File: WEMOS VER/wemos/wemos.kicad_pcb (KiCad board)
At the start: 2 copper layers, 50 x 50 mm, 15 parts, among them J1 9V BATT, J2 MOTOR 1, J3 MOTOR 2, SW1 RESET, SW2 ON/OFF, U1 WeMos D1 Mini, U2 L7805, U3 L293D

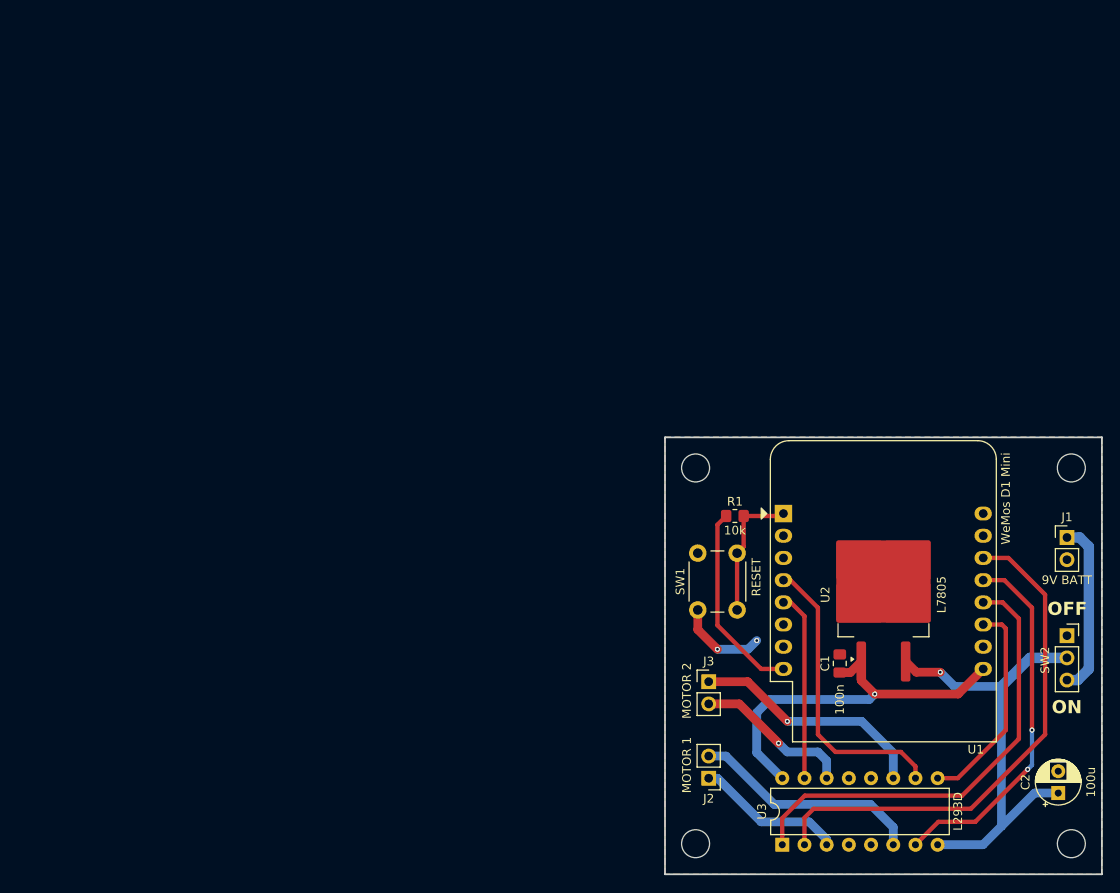
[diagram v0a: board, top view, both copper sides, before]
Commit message: A LOT OF WORK
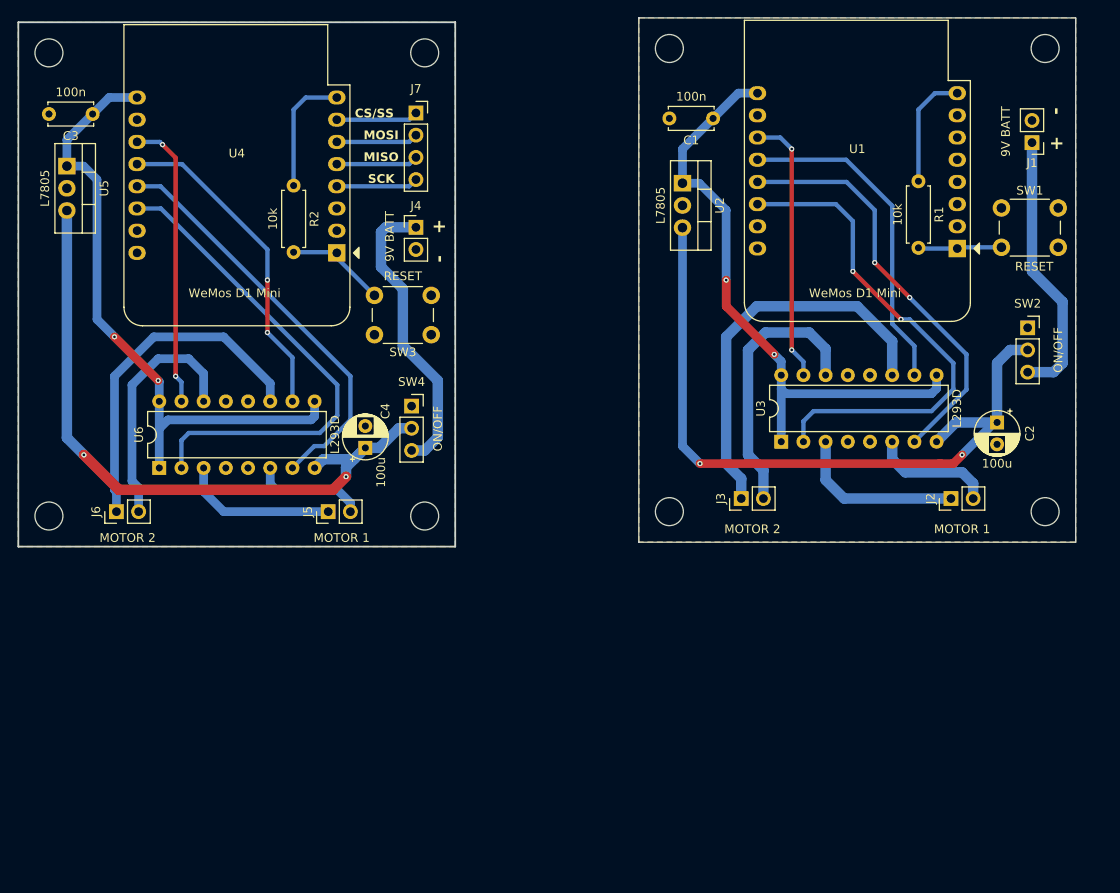
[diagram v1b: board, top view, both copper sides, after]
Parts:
- added C3: 100n, Capacitor_THT:C_Disc_D5.0mm_W2.5mm_P5.00mm, F.Cu at (49.5, 48.0)
- added C4: 100u, Capacitor_THT:CP_Radial_D5.0mm_P2.50mm, F.Cu at (80.7, 86.2)
- added H5: MountingHole, MountingHole:MountingHole_3.2mm_M3, F.Cu at (44.5, 41.0)
- added H6: MountingHole, MountingHole:MountingHole_3.2mm_M3, F.Cu at (87.5, 41.0)
- added H7: MountingHole, MountingHole:MountingHole_3.2mm_M3, F.Cu at (44.5, 94.0)
- added H8: MountingHole, MountingHole:MountingHole_3.2mm_M3, F.Cu at (87.5, 94.0)
- added J4: 9V BATT, Connector_PinHeader_2.54mm:PinHeader_1x02_P2.54mm_Vertical, F.Cu at (86.5, 61.0)
- added J5: MOTOR 1, Connector_PinHeader_2.54mm:PinHeader_1x02_P2.54mm_Vertical, F.Cu at (76.5, 93.5)
- added J6: MOTOR 2, Connector_PinHeader_2.54mm:PinHeader_1x02_P2.54mm_Vertical, F.Cu at (52.2, 93.5)
- added J7: Conn_01x04_Pin, Connector_PinSocket_2.54mm:PinSocket_1x04_P2.54mm_Vertical, F.Cu at (86.5, 47.9)
- added R2: 10k, Resistor_THT:R_Axial_DIN0207_L6.3mm_D2.5mm_P7.62mm_Horizontal, F.Cu at (72.5, 56.2)
- added SW3: RESET, Button_Switch_THT:SW_PUSH_6mm, F.Cu at (88.2, 73.2)
- added SW4: ON/OFF, Connector_PinSocket_2.54mm:PinSocket_1x03_P2.54mm_Vertical, F.Cu at (86.0, 81.4)
- added U4: WeMos D1 Mini, Module:WEMOS_D1_mini_light, F.Cu at (77.4, 63.9)
- added U5: L7805, Package_TO_SOT_THT:TO-220-3_Vertical, F.Cu at (46.6, 54.0)
- added U6: L293D, Package_DIP:DIP-16_W7.62mm, F.Cu at (57.1, 88.5)
- C1: footprint Capacitor_SMD:C_0805_2012Metric_Pad1.18x1.45mm_HandSolder -> Capacitor_THT:C_Disc_D5.0mm_W2.5mm_P5.00mm
- R1: footprint Resistor_SMD:R_0805_2012Metric_Pad1.20x1.40mm_HandSolder -> Resistor_THT:R_Axial_DIN0207_L6.3mm_D2.5mm_P7.62mm_Horizontal
- U2: footprint Package_TO_SOT_SMD:TO-263-2 -> Package_TO_SOT_THT:TO-220-3_Vertical
- moved C1 64.0 mm to (120.5, 48.5), turned to 180 degrees
- moved SW1 57.7 mm to (153.5, 58.8), turned to 0 degrees
- moved U2 52.4 mm to (117.0, 55.9), turned to -90 degrees
- moved H1 48.1 mm to (115.5, 40.5)
- moved H2 48.1 mm to (158.5, 40.5)
- moved U3 46.1 mm to (128.3, 85.5)
- moved J1 45.4 mm to (157.0, 51.3), turned to 180 degrees
- moved R1 43.7 mm to (144.0, 55.7), turned to -90 degrees
- moved C2 43.0 mm to (153.0, 83.3), turned to -90 degrees
- moved J2 42.3 mm to (147.7, 92.0), turned to 90 degrees
- moved H3 38.1 mm to (115.5, 93.5)
- moved H4 38.1 mm to (158.5, 93.5)
- moved U1 36.3 mm to (148.4, 63.4), turned to 180 degrees
- moved SW2 35.5 mm to (156.5, 72.5)
- moved J3 21.3 mm to (123.7, 92.0), turned to 90 degrees
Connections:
- U1 pad 4: Net-(U1-SCK/D5) -> unconnected-(U1-SCK/D5-Pad4)
- U1 pad 5: Net-(U1-MISO/D6) -> unconnected-(U1-MISO/D6-Pad5)
- U3 pad 1: Net-(U1-D3) -> +5V
- U3 pad 10: Net-(U1-SCK/D5) -> Net-(U1-D3)
- U3 pad 15: Net-(U1-MISO/D6) -> Net-(U1-D4)
- U3 pad 9: Net-(U1-D4) -> +5V
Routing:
- net +9VA: track 0.00 -> 78.2 mm, vias 0 -> 2
- net +5VA: track 0.00 -> 73.2 mm, vias 0 -> 2
- net Net-(U4-SCL/D1): track 0.00 -> 57.0 mm
- net Net-(U4-SDA/D2): track 0.00 -> 47.3 mm
- net Net-(J6-Pin_1): track 0.00 -> 39.5 mm
- net Net-(U4-D3): track 0.00 -> 37.5 mm, vias 0 -> 2
- net Net-(J4-Pin_1): track 0.00 -> 34.0 mm
- net Net-(U1-SCK/D5): track 33.8 -> 0.00 mm
- net Net-(U4-D4): track 0.00 -> 33.3 mm, vias 0 -> 2
- net +9V: track 53.2 -> 82.5 mm, vias 1 -> 2
- net Net-(J6-Pin_2): track 0.00 -> 28.1 mm
- net +5V: track 44.0 -> 70.3 mm, vias 1 -> 2
- net Net-(U1-MISO/D6): track 21.6 -> 0.00 mm
- net Net-(J5-Pin_1): track 0.00 -> 17.9 mm
- net Net-(J3-Pin_1): track 27.4 -> 45.2 mm, vias 1 -> 0
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- added copper zone on B.Cu, net GND1
- added copper zone on F.Cu, net GND1
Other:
- board size 50 x 50 mm -> 121 x 60.5 mm
- board text added: "+"
- board text added: "-"
- board text added: "CS/SS"
- board text added: "MISO"
- board text added: "MOSI"
- board text added: "SCK"
- board text removed: "OFF"
- board text removed: "ON"
